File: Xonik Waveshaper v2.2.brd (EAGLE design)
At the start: 55.9 x 21 mm, 78 parts, among them IC1 TL074JT, IC2 TL074JT, IC3 TL074JT, IC4 TL072JT, IC5 4013T, IC6 LM311T, T1 2n3904

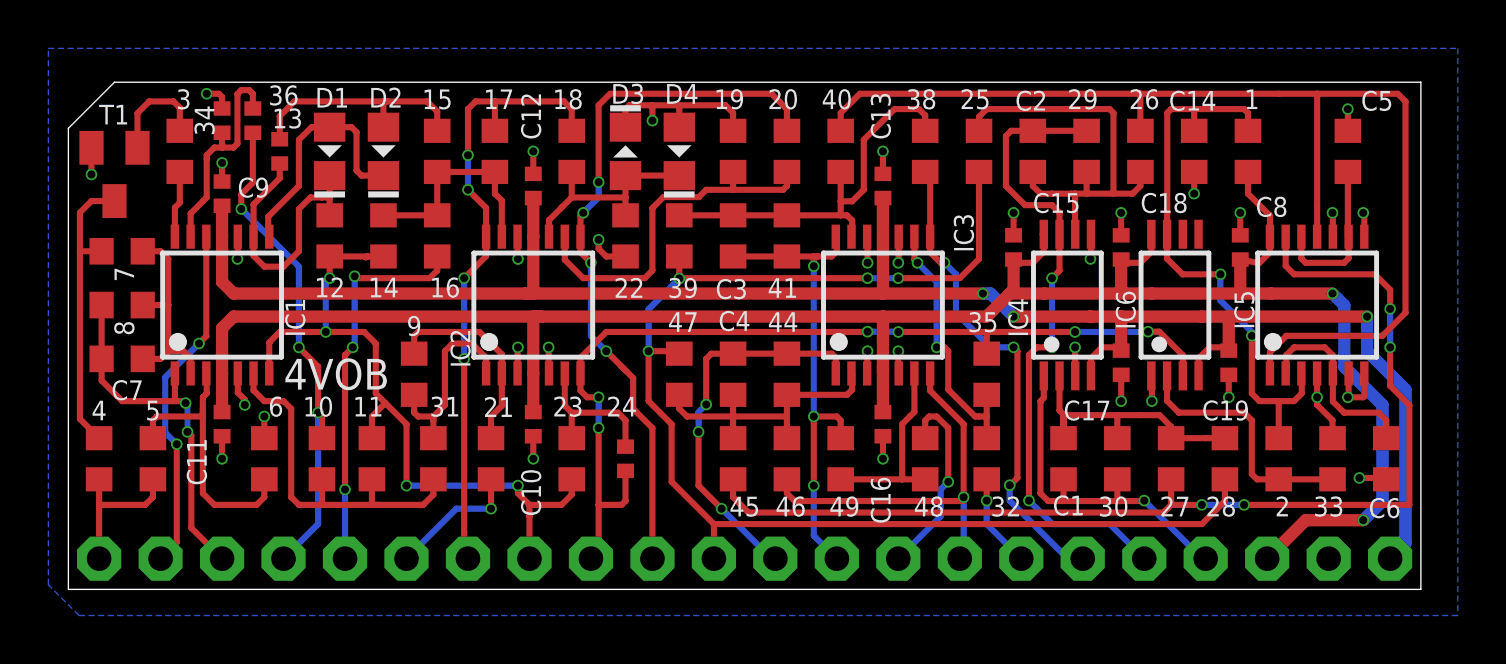
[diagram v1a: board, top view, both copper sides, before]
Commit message: Checked with JLCPCB
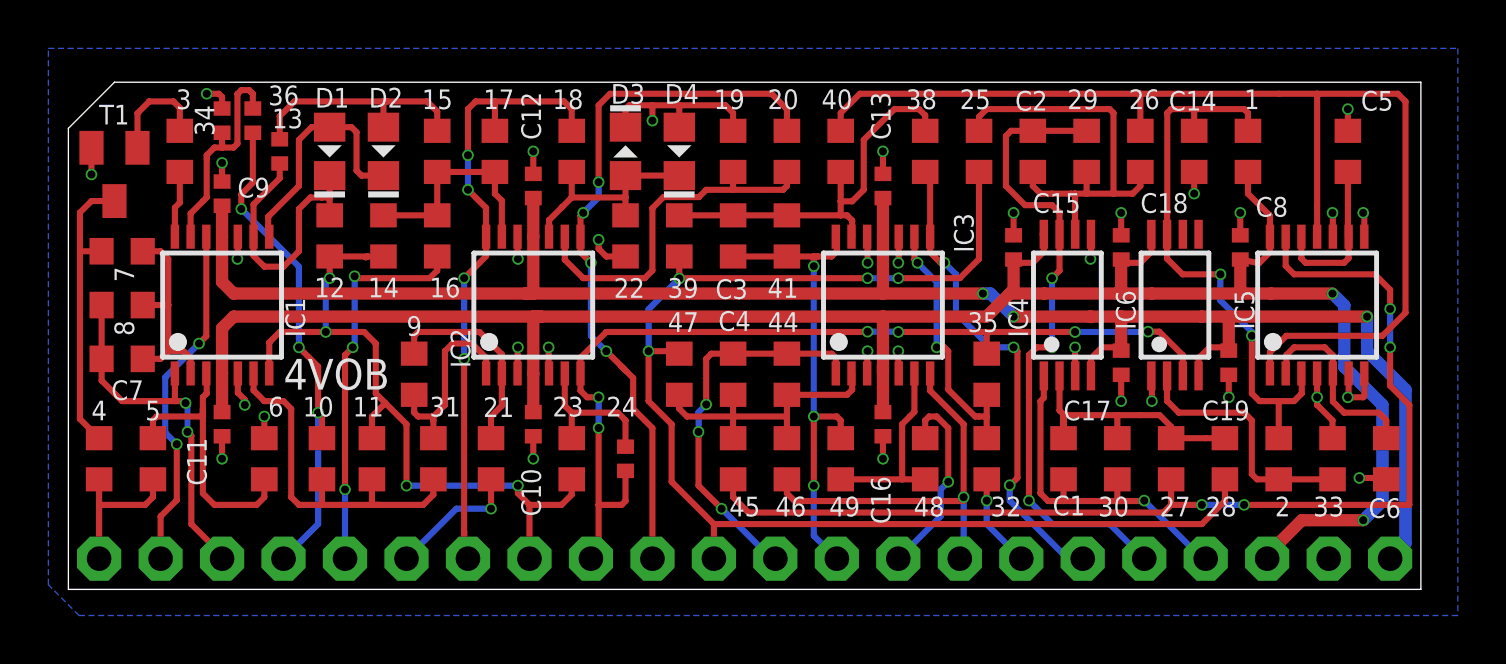
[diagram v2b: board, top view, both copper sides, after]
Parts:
- moved X1 11.4 mm to (27.9, 1.27)
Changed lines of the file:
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@@
 <attribute name="VALUE" x="9.525" y="18.7325" size="1.27" layer="27" rot="R90"/>
 </element>
-<element name="X1" library="joakim" package="MA22N-1J" value="" x="16.51" y="1.27" smashed="yes">
-<attribute name="VALUE" x="54.61" y="-1.651" size="1.27" layer="27" ratio="10"/>
+<element name="X1" library="joakim" package="MA22N-1J" value="" x="27.94" y="1.27" smashed="yes">
+<attribute name="VALUE" x="66.04" y="-1.651" size="1.27" layer="27" ratio="10"/>
 </element>
 </elements>
@@
 <contactref element="5" pad="2"/>
 <wire x1="1.27" y1="4.5475" x2="1.27" y2="3.4925" width="0.254" layer="1"/>
+<wire x1="1.27" y1="3.4925" x2="1.27" y2="1.27" width="0.254" layer="1"/>
 <wire x1="1.27" y1="3.4925" x2="3.175" y2="3.4925" width="0.254" layer="1"/>
 <wire x1="3.4925" y1="3.81" x2="3.175" y2="3.4925" width="0.254" layer="1"/>
 <wire x1="3.4925" y1="3.81" x2="3.4925" y2="4.5475" width="0.254" layer="1"/>
-<wire x1="1.27" y1="1.27" x2="1.27" y2="3.4925" width="0.254" layer="1"/>
 <contactref element="X1" pad="1"/>
 </signal>
@@
 <wire x1="4.92125" y1="7.62" x2="4.92125" y2="6.50875" width="0.254" layer="16"/>
 <via x="4.92125" y="6.50875" extent="1-16" drill="0.3302"/>
+<wire x1="6.35" y1="1.42875" x2="5.08" y2="2.69875" width="0.254" layer="1"/>
+<wire x1="6.35" y1="1.42875" x2="6.35" y2="1.27" width="0.254" layer="1"/>
 <wire x1="4.92125" y1="6.50875" x2="5.08" y2="6.35" width="0.254" layer="1"/>
-<wire x1="5.08" y1="2.54" x2="6.35" y2="1.27" width="0.254" layer="1"/>
-<wire x1="5.08" y1="6.35" x2="5.08" y2="2.54" width="0.254" layer="1"/>
+<wire x1="5.08" y1="6.35" x2="5.08" y2="2.69875" width="0.254" layer="1"/>
 <wire x1="4.4" y1="8.9225" x2="4.4" y2="7.82375" width="0.254" layer="1"/>
 <wire x1="4.4" y1="7.82375" x2="4.445" y2="7.77875" width="0.254" layer="1"/>
@@
 <wire x1="18.57375" y1="4.28625" x2="13.97" y2="4.28625" width="0.254" layer="16"/>
 <via x="13.97" y="4.28625" extent="1-16" drill="0.3302"/>
-<wire x1="19.05" y1="1.27" x2="19.05" y2="3.01625" width="0.254" layer="1"/>
-<wire x1="19.05" y1="3.01625" x2="19.05" y2="3.4925" width="0.254" layer="1"/>
+<wire x1="19.05" y1="1.27" x2="19.05" y2="3.4925" width="0.254" layer="1"/>
 <wire x1="10.63625" y1="10.63625" x2="12.22375" y2="10.63625" width="0.254" layer="1"/>
 <wire x1="12.7" y1="8.09625" x2="13.096875" y2="7.699375" width="0.254" layer="1"/>
@@
 <via x="39.6875" y="3.6703" extent="1-16" drill="0.3302"/>
 <wire x1="39.6875" y1="3.6703" x2="40.65905" y2="2.69875" width="0.254" layer="16"/>
-<wire x1="43.02125" y1="2.69875" x2="44.45" y2="1.27" width="0.254" layer="16"/>
-<wire x1="40.65905" y1="2.69875" x2="43.02125" y2="2.69875" width="0.254" layer="16"/>
+<wire x1="43.03968125" y1="2.68031875" x2="43.03434375" y2="2.69875" width="0.254" layer="16"/>
+<wire x1="43.03968125" y1="2.68031875" x2="44.45" y2="1.27" width="0.254" layer="16"/>
+<wire x1="40.65905" y1="2.69875" x2="43.03434375" y2="2.69875" width="0.254" layer="16"/>
 <contactref element="X1" pad="18"/>
 </signal>
@@
 <wire x1="44.45" y1="3.65125" x2="44.45" y2="3.6703" width="0.254" layer="1"/>
 <via x="44.45" y="3.6703" extent="1-16" drill="0.3302"/>
-<wire x1="46.99" y1="1.27" x2="46.8503" y2="1.27" width="0.254" layer="16"/>
-<wire x1="46.8503" y1="1.27" x2="44.45" y2="3.6703" width="0.254" layer="16"/>
+<wire x1="46.99" y1="1.27" x2="46.961484375" y2="1.158815625" width="0.254" layer="16"/>
+<wire x1="46.961484375" y1="1.158815625" x2="44.45" y2="3.6703" width="0.254" layer="16"/>
 <contactref element="X1" pad="19"/>
 </signal>
@@
 <wire x1="30.7975" y1="13.35405" x2="30.7975" y2="13.755" width="0.254" layer="1"/>
 <via x="30.7975" y="4.28625" extent="1-16" drill="0.3302"/>
-<wire x1="30.7975" y1="2.2225" x2="31.75" y2="1.27" width="0.254" layer="16"/>
-<wire x1="30.7975" y1="4.28625" x2="30.7975" y2="2.2225" width="0.254" layer="16"/>
 <contactref element="X1" pad="13"/>
+<wire x1="31.75" y1="1.27" x2="30.7975" y2="2.2225" width="0.254" layer="16"/>
+<wire x1="30.7975" y1="2.2225" x2="30.7975" y2="4.28625" width="0.254" layer="16"/>
 </signal>
 <signal name="-5V">
@@
 <wire x1="47.78375" y1="3.65125" x2="47.78375" y2="4.5475" width="0.254" layer="1"/>
 <wire x1="47.78375" y1="3.65125" x2="46.83125" y2="2.69875" width="0.254" layer="1"/>
-<wire x1="26.67" y1="2.69875" x2="46.83125" y2="2.69875" width="0.254" layer="1"/>
 <wire x1="37.62375" y1="17.2475" x2="37.62375" y2="13.6525" width="0.254" layer="1"/>
 <wire x1="36.83" y1="12.85875" x2="34.29" y2="12.85875" width="0.254" layer="1"/>
@@
 <wire x1="37.62375" y1="13.6525" x2="36.83" y2="12.85875" width="0.254" layer="1"/>
 <wire x1="23.97125" y1="7.77875" x2="24.92375" y2="6.82625" width="0.254" layer="1"/>
-<wire x1="24.92375" y1="4.445" x2="26.67" y2="2.69875" width="0.254" layer="1"/>
-<wire x1="24.92375" y1="6.82625" x2="24.92375" y2="4.445" width="0.254" layer="1"/>
-<wire x1="26.67" y1="2.69875" x2="26.67" y2="1.27" width="0.254" layer="1"/>
+<wire x1="24.92375" y1="4.445" x2="24.92375" y2="6.82625" width="0.254" layer="1"/>
 <contactref element="X1" pad="11"/>
+<wire x1="26.67" y1="1.27" x2="26.67" y2="2.69875" width="0.254" layer="1"/>
+<wire x1="46.83125" y1="2.69875" x2="26.67" y2="2.69875" width="0.254" layer="1"/>
+<wire x1="26.67" y1="2.69875" x2="24.92375" y2="4.445" width="0.254" layer="1"/>
 </signal>
 <signal name="SS2_TRIM_R">
@@
 <wire x1="36.98875" y1="6.82625" x2="35.605" y2="8.21" width="0.254" layer="1"/>
 <via x="36.98875" y="3.81" extent="1-16" drill="0.3302"/>
-<wire x1="36.98875" y1="1.42875" x2="36.83" y2="1.27" width="0.254" layer="16"/>
-<wire x1="36.98875" y1="3.81" x2="36.98875" y2="1.42875" width="0.254" layer="16"/>
+<wire x1="36.98875" y1="1.310953125" x2="36.83" y2="1.27" width="0.254" layer="16"/>
+<wire x1="36.98875" y1="3.81" x2="36.98875" y2="1.310953125" width="0.254" layer="16"/>
 <contactref element="X1" pad="15"/>
 </signal>
@@
 <wire x1="26.035" y1="4.28625" x2="26.9875" y2="3.33375" width="0.254" layer="1"/>
 <via x="26.9875" y="3.33375" extent="1-16" drill="0.3302"/>
-<wire x1="29.21" y1="1.27" x2="29.05125" y2="1.27" width="0.254" layer="16"/>
-<wire x1="29.05125" y1="1.27" x2="26.9875" y2="3.33375" width="0.254" layer="16"/>
+<wire x1="29.21" y1="1.27" x2="29.1775875" y2="1.1436625" width="0.254" layer="16"/>
+<wire x1="29.1775875" y1="1.1436625" x2="26.9875" y2="3.33375" width="0.254" layer="16"/>
 <contactref element="X1" pad="12"/>
 </signal>
@@
 <wire x1="16.35125" y1="9.525" x2="16.35125" y2="2.38125" width="0.254" layer="1"/>
 <wire x1="16.35125" y1="2.38125" x2="16.35125" y2="2.2225" width="0.254" layer="1"/>
-<wire x1="16.35125" y1="2.38125" x2="16.35125" y2="1.42875" width="0.254" layer="1"/>
-<wire x1="16.35125" y1="1.42875" x2="16.51" y2="1.27" width="0.254" layer="1"/>
+<wire x1="16.35125" y1="2.38125" x2="16.35125" y2="1.311190625" width="0.254" layer="1"/>
+<wire x1="16.35125" y1="1.311190625" x2="16.51" y2="1.27" width="0.254" layer="1"/>
 <contactref element="X1" pad="7"/>
 </signal>
@@
 <wire x1="52.7177" y1="11.7348" x2="52.7177" y2="9.1948" width="0.508" layer="16"/>
 <via x="53.49875" y="2.8575" extent="1-16" drill="0.3302"/>
-<wire x1="53.49875" y1="2.8575" x2="51.1175" y2="2.8575" width="0.508" layer="1"/>
-<wire x1="51.1175" y1="2.8575" x2="49.53" y2="1.27" width="0.508" layer="1"/>
+<wire x1="53.49875" y1="2.8575" x2="50.95875" y2="2.8575" width="0.508" layer="1"/>
+<wire x1="50.95875" y1="2.8575" x2="49.53" y2="1.42875" width="0.508" layer="1"/>
+<wire x1="49.53" y1="1.42875" x2="49.53" y2="1.27" width="0.508" layer="1"/>
 <contactref element="X1" pad="20"/>
 </signal>
@@
 <via x="38.89375" y="4.3053" extent="1-16" drill="0.3302"/>
 <wire x1="39.21125" y1="9.8425" x2="39.21125" y2="4.60375" width="0.254" layer="1"/>
-<wire x1="41.29405" y1="1.27" x2="41.91" y2="1.27" width="0.254" layer="16"/>
-<wire x1="41.29405" y1="1.27" x2="38.89375" y2="3.6703" width="0.254" layer="16"/>
 <wire x1="38.89375" y1="4.3053" x2="38.89375" y2="3.6703" width="0.254" layer="16"/>
 <contactref element="X1" pad="17"/>
+<wire x1="38.89375" y1="3.6703" x2="41.29405" y2="1.27" width="0.254" layer="16"/>
+<wire x1="41.29405" y1="1.27" x2="41.91" y2="1.27" width="0.254" layer="16"/>
 </signal>
 <signal name="-12V">
@@
 <wire x1="55.245" y1="8.255" x2="53.6575" y2="9.8425" width="0.508" layer="16"/>
 <wire x1="55.245" y1="8.255" x2="55.245" y2="1.905" width="0.508" layer="16"/>
-<wire x1="55.245" y1="1.905" x2="54.61" y2="1.27" width="0.508" layer="16"/>
+<wire x1="54.61" y1="1.27" x2="55.245" y2="1.905" width="0.508" layer="16"/>
 <wire x1="43.4975" y1="9.86625" x2="43.4825" y2="10.00125" width="0.254" layer="1"/>
 <wire x1="43.4825" y1="10.00125" x2="42.70375" y2="10.00125" width="0.254" layer="1"/>
@@
 <wire x1="4.47773125" y1="5.99976875" x2="4.00148125" y2="6.47601875" width="0.254" layer="16"/>
 <via x="4.47773125" y="5.99976875" extent="1-16" drill="0.3302"/>
-<wire x1="4.47773125" y1="5.99976875" x2="4.47773125" y2="1.93773125" width="0.254" layer="1"/>
-<wire x1="4.47773125" y1="1.93773125" x2="3.81" y2="1.27" width="0.254" layer="1"/>
+<wire x1="4.47773125" y1="5.99976875" x2="4.47773125" y2="3.68398125" width="0.254" layer="1"/>
+<wire x1="3.81" y1="1.27" x2="3.81" y2="3.01625" width="0.254" layer="1"/>
+<wire x1="4.47773125" y1="3.68398125" x2="3.81" y2="3.01625" width="0.254" layer="1"/>
 <wire x1="4.00148125" y1="6.47601875" x2="4.00148125" y2="8.76398125" width="0.254" layer="16"/>
 <wire x1="4.00148125" y1="8.76398125" x2="5.3975" y2="10.16" width="0.254" layer="16"/>
